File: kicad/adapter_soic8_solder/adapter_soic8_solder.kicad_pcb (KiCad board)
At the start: 2 copper layers, 48 x 20 mm, 3 parts, among them J1 Conn_02x07_Odd_Even, J2 Conn_02x07_Odd_Even, U1 AT45DB

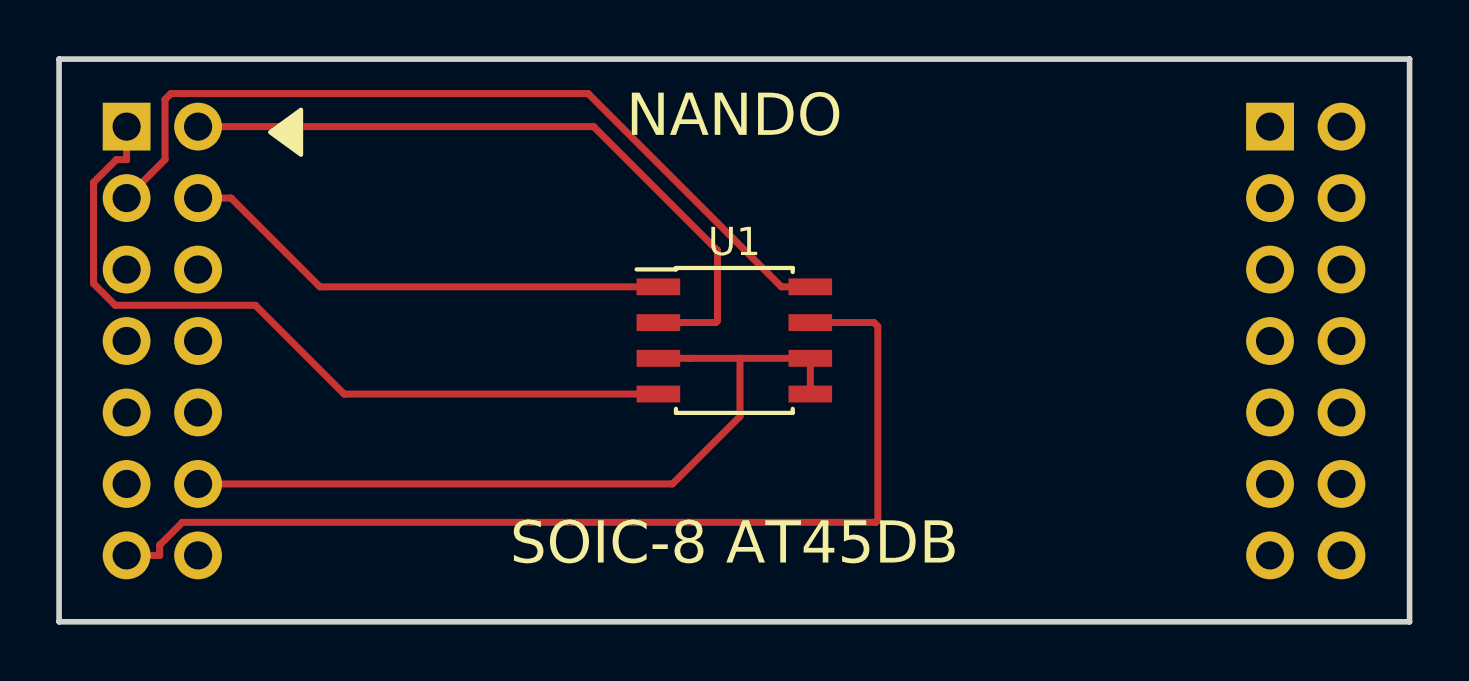
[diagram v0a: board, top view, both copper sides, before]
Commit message: update PCB design and cleanup KiCad files
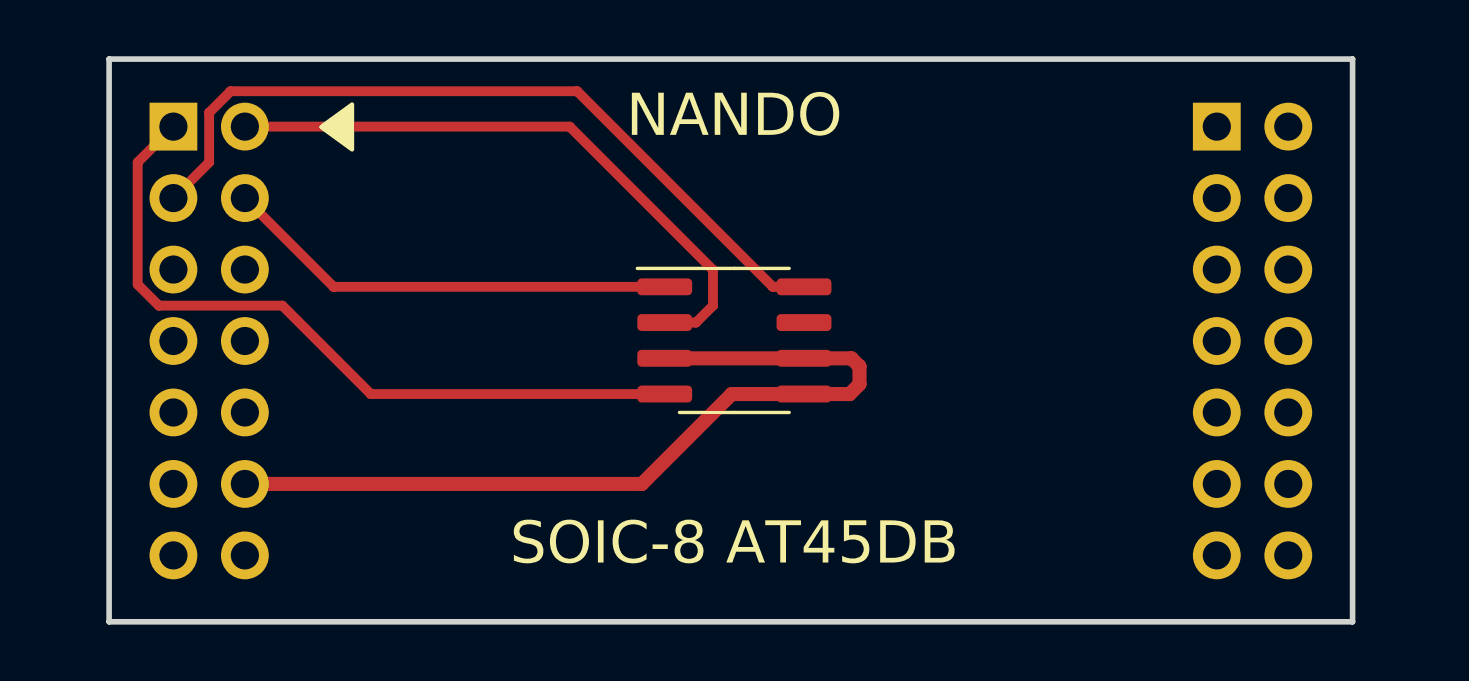
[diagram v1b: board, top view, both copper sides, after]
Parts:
- J1, J2: footprint lib_fp:PinSocket_2x07_P2.54mm_Vertical -> Connector_PinSocket_2.54mm:PinSocket_2x07_P2.54mm_Vertical
- U1: footprint lib_fp:SOIC-8_3.9x4.9mm_P1.27mm -> Package_SO:SOIC-8_3.9x4.9mm_P1.27mm
- moved J2 1.89 mm to (174.0, 79.4)
- moved J1 1.66 mm to (136.9, 79.4)
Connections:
- J1 pad 10: Net-(J1-Pad10) -> unconnected-(J1-Pin_10-Pad10)
- J1 pad 11: Net-(J1-Pad11) -> unconnected-(J1-Pin_11-Pad11)
- J1 pad 14: Net-(J1-Pad14) -> unconnected-(J1-Pin_14-Pad14)
- J1 pad 5: Net-(J1-Pad5) -> unconnected-(J1-Pin_5-Pad5)
- J1 pad 6: Net-(J1-Pad6) -> unconnected-(J1-Pin_6-Pad6)
- J1 pad 7: Net-(J1-Pad7) -> unconnected-(J1-Pin_7-Pad7)
- J1 pad 8: Net-(J1-Pad8) -> unconnected-(J1-Pin_8-Pad8)
- J1 pad 9: Net-(J1-Pad9) -> unconnected-(J1-Pin_9-Pad9)
- J2 pad 1: Net-(J2-Pad1) -> GNDD
- J2 pad 10: Net-(J2-Pad10) -> unconnected-(J2-Pin_10-Pad10)
- J2 pad 11: Net-(J2-Pad11) -> unconnected-(J2-Pin_11-Pad11)
- J2 pad 12: Net-(J2-Pad12) -> unconnected-(J2-Pin_12-Pad12)
- J2 pad 13: Net-(J2-Pad13) -> GNDD
- J2 pad 14: Net-(J2-Pad14) -> unconnected-(J2-Pin_14-Pad14)
- J2 pad 2: Net-(J2-Pad2) -> unconnected-(J2-Pin_2-Pad2)
- J2 pad 3: Net-(J2-Pad3) -> unconnected-(J2-Pin_3-Pad3)
- J2 pad 4: Net-(J2-Pad4) -> unconnected-(J2-Pin_4-Pad4)
- J2 pad 5: Net-(J2-Pad5) -> unconnected-(J2-Pin_5-Pad5)
- J2 pad 6: Net-(J2-Pad6) -> unconnected-(J2-Pin_6-Pad6)
- J2 pad 7: Net-(J2-Pad7) -> unconnected-(J2-Pin_7-Pad7)
- J2 pad 8: Net-(J2-Pad8) -> unconnected-(J2-Pin_8-Pad8)
- J2 pad 9: Net-(J2-Pad9) -> unconnected-(J2-Pin_9-Pad9)
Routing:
- net GNDD: track 36.8 -> 0.47 mm
- net SCK: track 24.9 -> 22.0 mm
- net SO: track 29.9 -> 27.9 mm
- net +3V3: track 29.0 -> 31.0 mm
- net CS: track 28.0 -> 26.5 mm
- net SI: track 17.7 -> 16.2 mm
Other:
- board size 48 x 20 mm -> 44.2 x 20 mm
- net class Default removed
- rule pad_to_mask_clearance: 0.051 -> 0.05
- rule solder_mask_min_width: 0.25 -> 0.1
